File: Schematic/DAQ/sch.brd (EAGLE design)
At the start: 108.9 x 87.6 mm, 46 parts, among them IC1 MCP23S17SP, IC2 MCP23S17SP, IC3 MCP23S17SP, IC4 74LS165N, U1 ATMEGA328P-PU

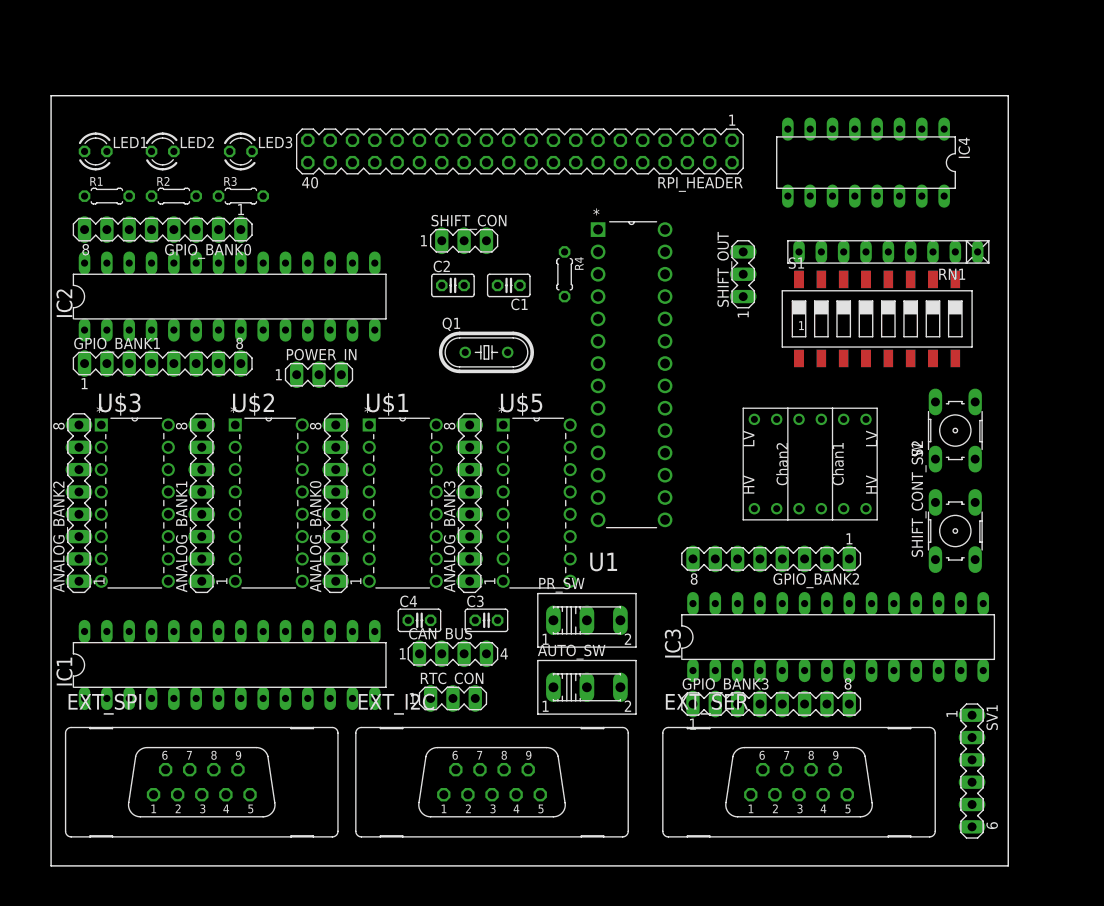
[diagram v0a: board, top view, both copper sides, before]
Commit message: Started board
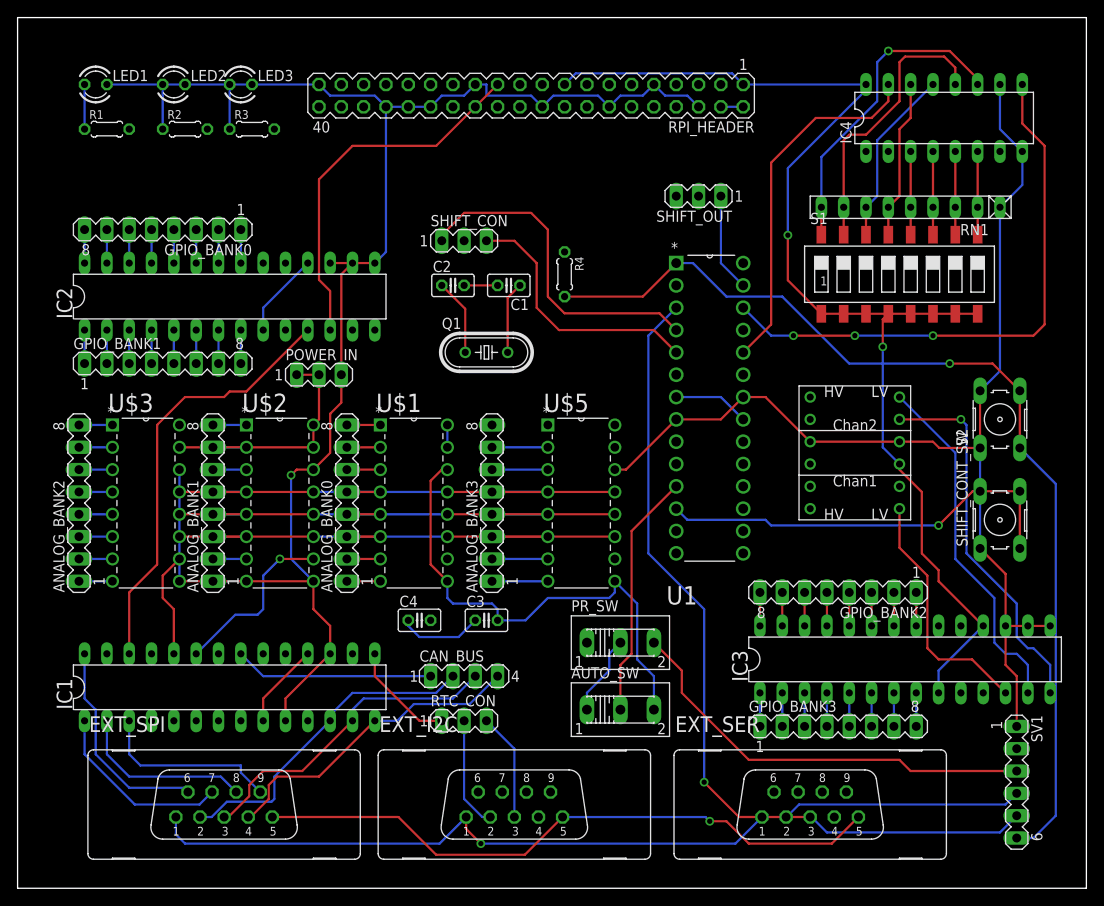
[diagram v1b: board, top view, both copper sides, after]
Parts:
- moved U$4 19.2 mm to (97.8, 54.6), turned to 180 degrees
- moved IC4 10.2 mm to (101.6, 85.1), turned to 0 degrees
- moved SHIFT_OUT 10.2 mm to (73.7, 76.2), turned to 180 degrees
- moved U1 9.67 mm to (78.7, 35.6)
- moved GPIO_BANK2 8.52 mm to (89.5, 31.1)
- moved IC3 8.03 mm to (97.2, 23.5)
- moved GPIO_BANK3 8.03 mm to (89.5, 15.9)
- moved LED2 7.73 mm to (14.0, 88.9)
- moved R2 7.73 mm to (15.2, 83.8)
- moved R3 7.73 mm to (22.9, 83.8)
- moved LED1 7.62 mm to (5.08, 88.9)
- moved LED3 7.62 mm to (21.6, 88.9)
- moved R1 7.62 mm to (6.35, 83.8)
- moved RPI_HEADER 6.48 mm to (54.6, 87.6)
- moved RN1 5.68 mm to (97.8, 74.9)
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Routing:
- net GND: track 0.00 -> 388.5 mm, vias 0 -> 1
- net 3V3: track 0.00 -> 154.1 mm, vias 0 -> 2
- net PR_RST: track 0.00 -> 114.9 mm, vias 0 -> 1
- net DAQ_SCK: track 0.00 -> 107.9 mm
- net DAQ_RX: track 0.00 -> 96.6 mm, vias 0 -> 1
- net DAQ_MISO: track 0.00 -> 78.6 mm, vias 0 -> 1
- net DAQ_MOSI: track 0.00 -> 77.2 mm
- net N$19: track 0.00 -> 73.6 mm, vias 0 -> 1
- net N$18: track 0.00 -> 72.7 mm, vias 0 -> 1
- net SH_OUT: track 0.00 -> 64.5 mm, vias 0 -> 3
- net N$32: track 0.00 -> 49.5 mm
- net N$31: track 0.00 -> 49.5 mm
- net N$30: track 0.00 -> 49.5 mm
- net GPIO_CS0: track 0.00 -> 49.0 mm
- net PR_VCC: track 0.00 -> 48.8 mm
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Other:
- board size 108.9 x 87.6 mm -> 121.6 x 99.1 mm
